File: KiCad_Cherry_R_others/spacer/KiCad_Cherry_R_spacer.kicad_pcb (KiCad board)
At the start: 2 copper layers, 138.1 x 100 mm, 15 parts

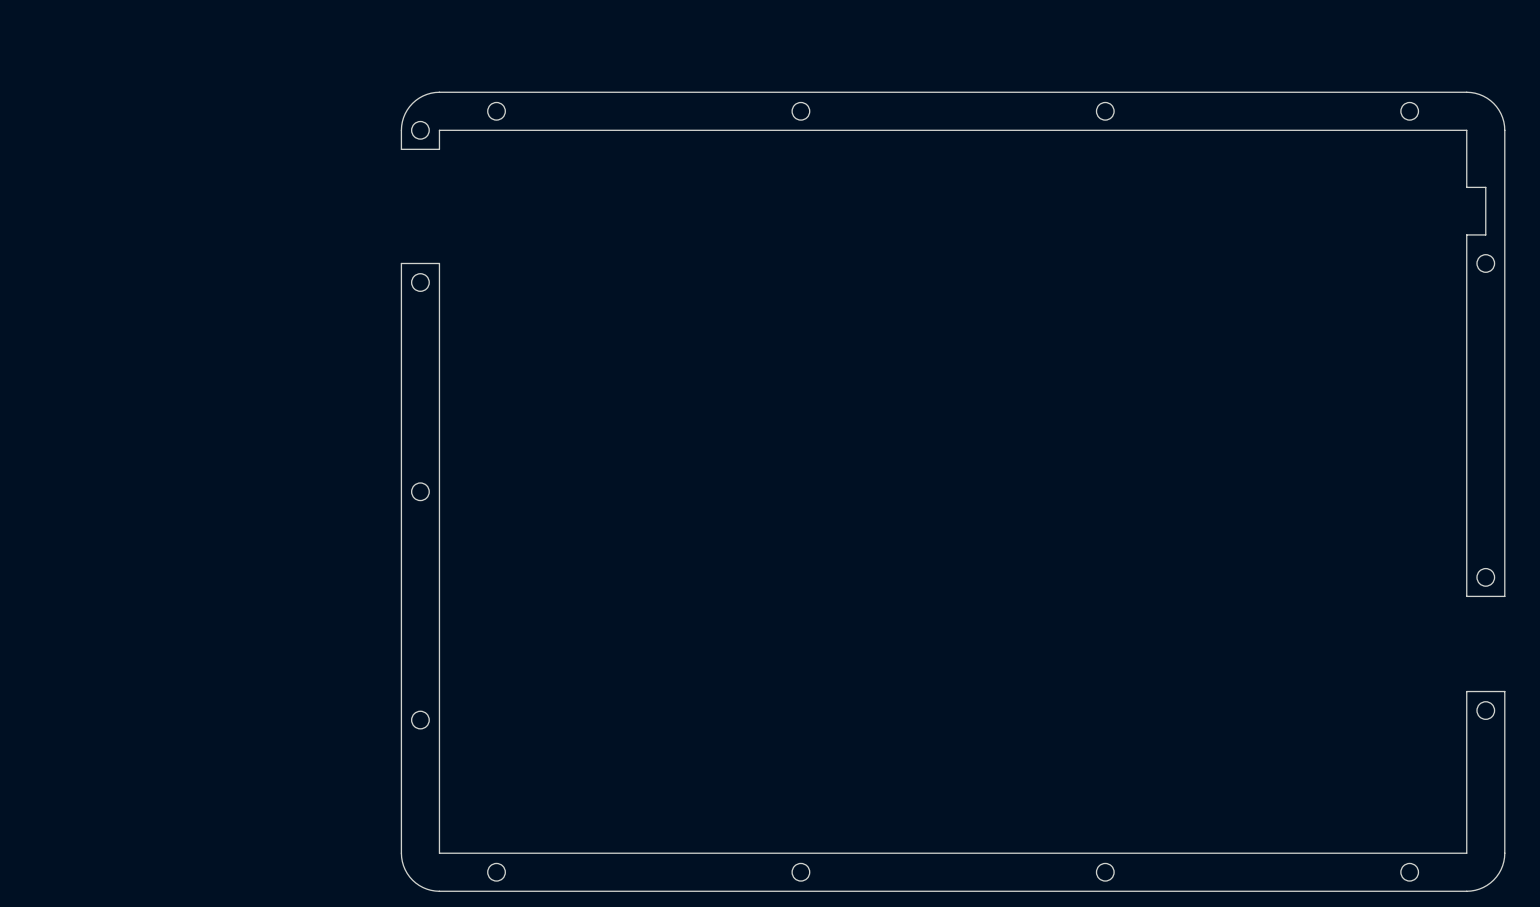
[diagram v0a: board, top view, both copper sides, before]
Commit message: feat: ガワがすべて完成
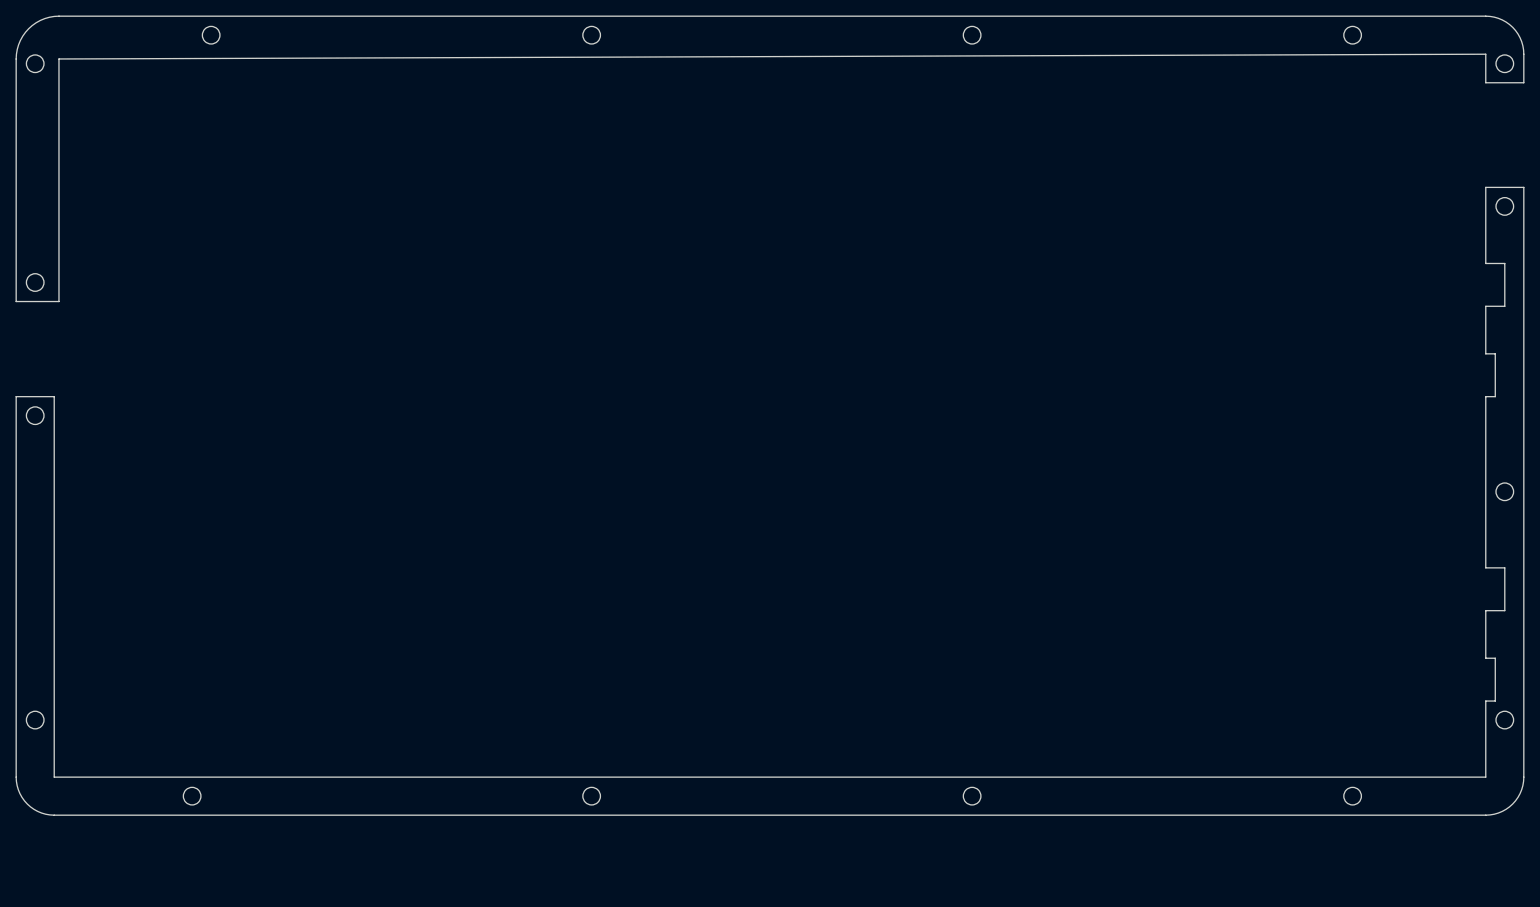
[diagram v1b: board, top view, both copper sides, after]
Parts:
- removed H10, H12, H13, H14, H2 (x6), H3, H4, H7, H8, H9: MountingHole_2.2mm_M2, MountingHole:MountingHole_2.2mm_M2
- added REF**: MountingHole_2.2mm_M2, MountingHole:MountingHole_2.2mm_M2, F.Cu at (35.1, 41.7)
- added REF**: MountingHole_2.2mm_M2, MountingHole:MountingHole_2.2mm_M2, F.Cu at (152.4, 38.1)
- added REF**: MountingHole_2.2mm_M2, MountingHole:MountingHole_2.2mm_M2, F.Cu at (104.8, 133.3)
- added REF**: MountingHole_2.2mm_M2, MountingHole:MountingHole_2.2mm_M2, F.Cu at (35.1, 69.1)
- added REF**: MountingHole_2.2mm_M2, MountingHole:MountingHole_2.2mm_M2, F.Cu at (152.4, 133.3)
- added REF**: MountingHole_2.2mm_M2, MountingHole:MountingHole_2.2mm_M2, F.Cu at (104.8, 38.1)
- added REF**: MountingHole_2.2mm_M2, MountingHole:MountingHole_2.2mm_M2, F.Cu at (200.0, 133.3)
- added REF**: MountingHole_2.2mm_M2, MountingHole:MountingHole_2.2mm_M2, F.Cu at (200.0, 38.1)
- added REF**: MountingHole_2.2mm_M2, MountingHole:MountingHole_2.2mm_M2, F.Cu at (219.1, 95.2)
- added REF**: MountingHole_2.2mm_M2, MountingHole:MountingHole_2.2mm_M2, F.Cu at (219.1, 41.7)
- added REF**: MountingHole_2.2mm_M2, MountingHole:MountingHole_2.2mm_M2, F.Cu at (57.1, 38.1)
- added REF**: MountingHole_2.2mm_M2, MountingHole:MountingHole_2.2mm_M2, F.Cu at (35.1, 123.8)
- added REF**: MountingHole_2.2mm_M2, MountingHole:MountingHole_2.2mm_M2, F.Cu at (219.1, 59.5)
- added REF**: MountingHole_2.2mm_M2, MountingHole:MountingHole_2.2mm_M2, F.Cu at (54.8, 133.3)
- added REF**: MountingHole_2.2mm_M2, MountingHole:MountingHole_2.2mm_M2, F.Cu at (219.1, 123.8)
- added REF**: MountingHole_2.2mm_M2, MountingHole:MountingHole_2.2mm_M2, F.Cu at (35.1, 85.7)
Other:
- board size 138.1 x 100 mm -> 188.7 x 100 mm
